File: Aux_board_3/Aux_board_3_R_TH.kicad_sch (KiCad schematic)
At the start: 40 parts, among them Q1 BSS138KJ, Q10 BSS84KJ, Q11 BSS138KJ, Q12 BSS84KJ, Q13 BSS138KJ, Q14 BSS84KJ, Q15 BSS138KJ, Q16 BSS84KJ, Q2 BSS84KJ, Q3 BSS138KJ, Q4 BSS84KJ, Q5 BSS138KJ, Q6 BSS84KJ, Q7 BSS138KJ, Q8 BSS84KJ, Q9 BSS138KJ

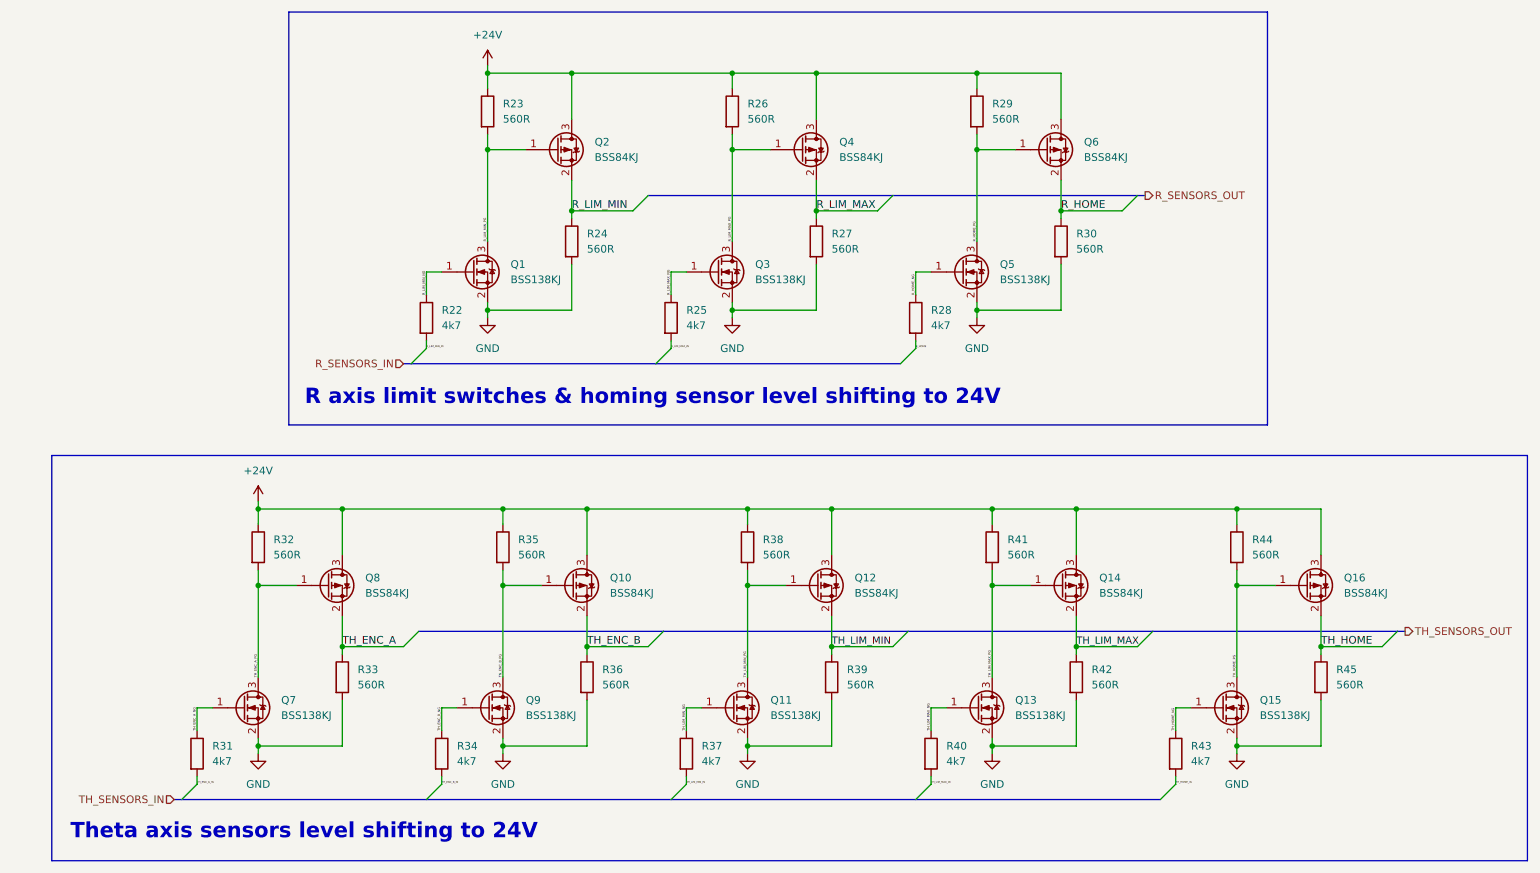
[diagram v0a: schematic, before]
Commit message: Board 3 layout started
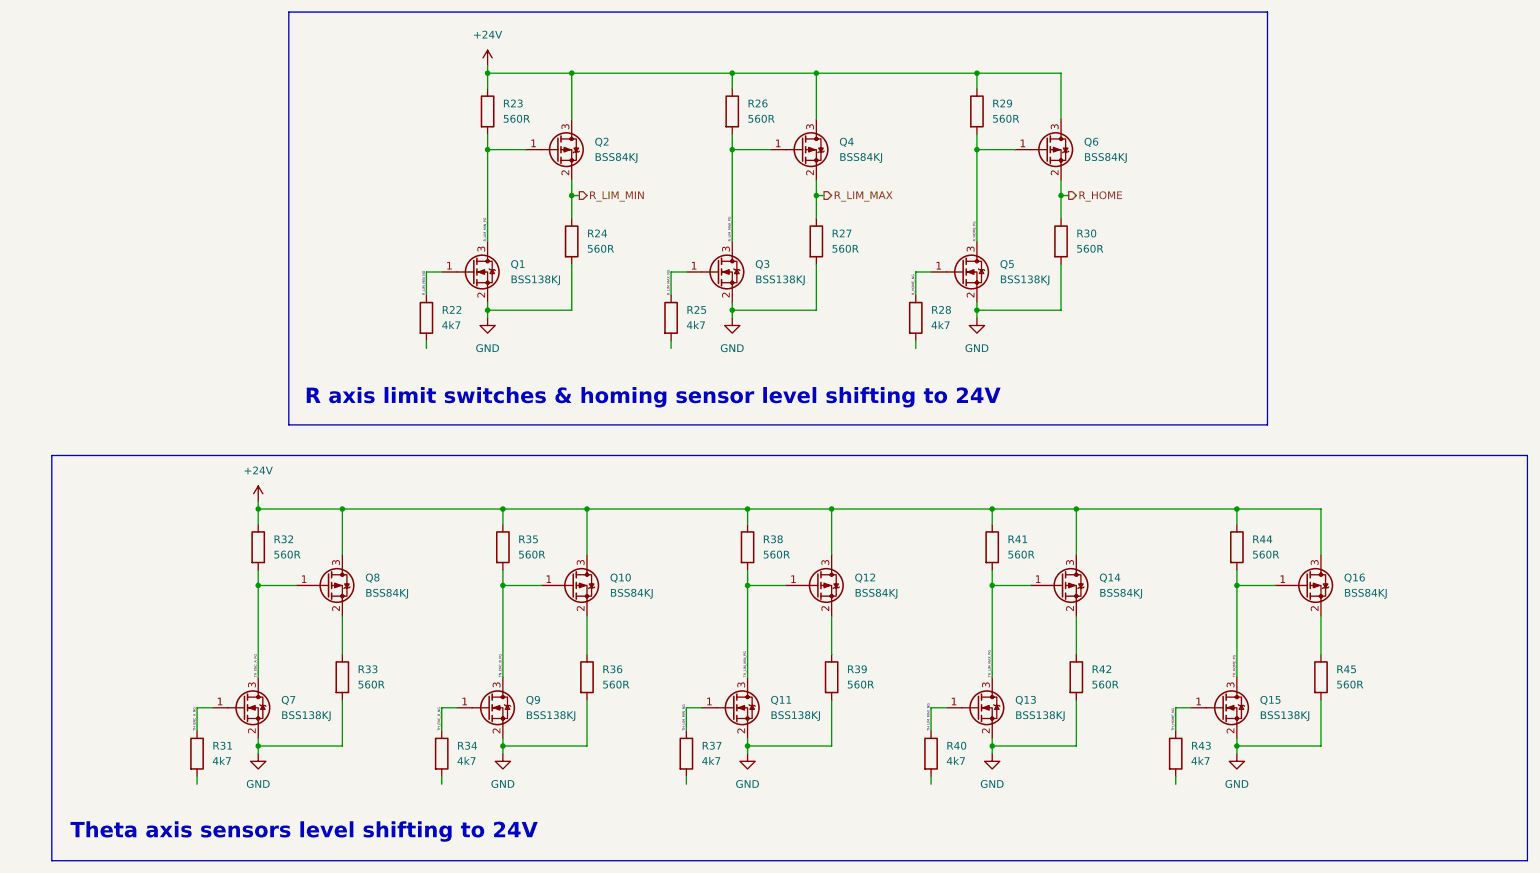
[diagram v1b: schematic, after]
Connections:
- net R_HOME: no longer R28.2
- net R_LIM_MAX_IN: no longer names the net of R25.2
- net R_LIM_MIN_IN: no longer names the net of R22.2
- net TH_ENC_A: no longer names the net of Q8.2 (S), R33.1
- net TH_ENC_A_IN: no longer names the net of R31.2
- net TH_ENC_B: no longer names the net of Q10.2 (S), R36.1
- net TH_ENC_B_IN: no longer names the net of R34.2
- net TH_HOME: no longer names the net of Q16.2 (S), R45.1
- net TH_HOME_IN: no longer names the net of R43.2
- net TH_LIM_MAX: no longer names the net of Q14.2 (S), R42.1
- net TH_LIM_MAX_IN: no longer names the net of R40.2
- net TH_LIM_MIN: no longer names the net of Q12.2 (S), R39.1
- net TH_LIM_MIN_IN: no longer names the net of R37.2
